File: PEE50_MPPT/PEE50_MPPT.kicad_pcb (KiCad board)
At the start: 2 copper layers, 125 x 125 mm, 174 parts, among them J1 Vout, J2 Conn_01x02_Female, J3 Conn_01x03_Female, J4 Conn_01x03_Female, J5 PV_IN1, J6 PV_IN1, J7 PV_IN1, J8 PV_IN1, Q1 BC547, Q2 BC547, Q3 BC547, Q4 BC547, SW1 SW_DIP_x01, U1 LM3480-3.3, U10 NTA4151PT1G, U11 CSD18514Q5A, U12 CSD18543Q3A, U13 TPS552882QRPMRQ1, U14 MAX44284FAUT+T, U15 MAX44284FAUT+T, U16 NTA4151PT1G, U17 CSD18514Q5A, U18 CSD18543Q3A, U19 TPS552882QRPMRQ1, U2 MSP430FR2353TDBT, U20 MAX44284FAUT+T, U21 MAX44284FAUT+T, U22 NTA4151PT1G, U23 CSD18514Q5A, U24 CSD18543Q3A, U25 TPS552882QRPMRQ1, U26 MAX44284FAUT+T, U27 MAX44284FAUT+T, U3 ADG706BRUZ, U4 NTA4151PT1G, U5 CSD18514Q5A, U6 CSD18543Q3A, U7 TPS552882QRPMRQ1, U8 MAX44284FAUT+T, U9 MAX44284FAUT+T

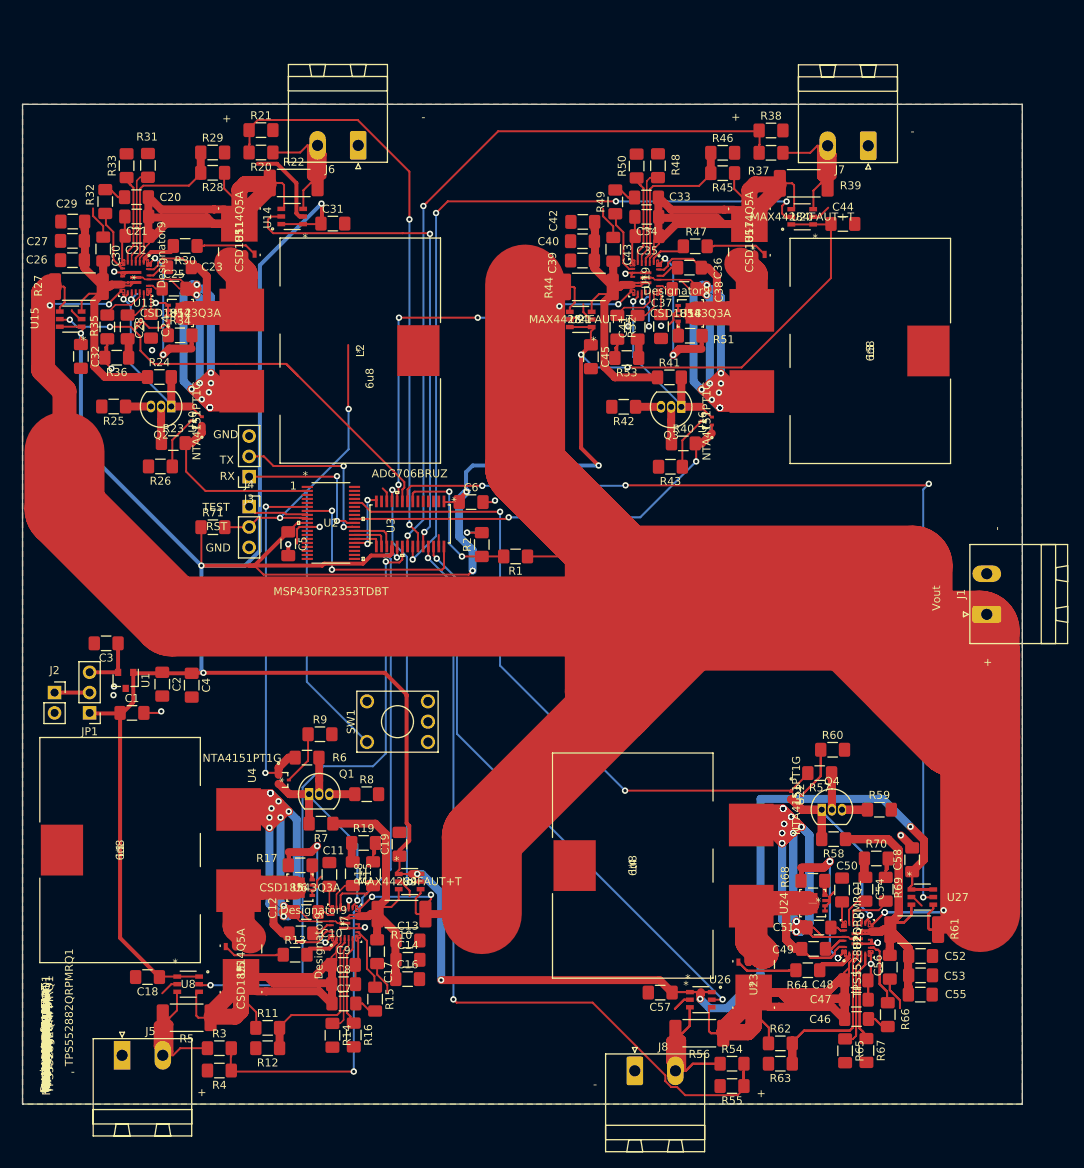
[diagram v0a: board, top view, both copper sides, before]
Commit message: PCB gedecimeert
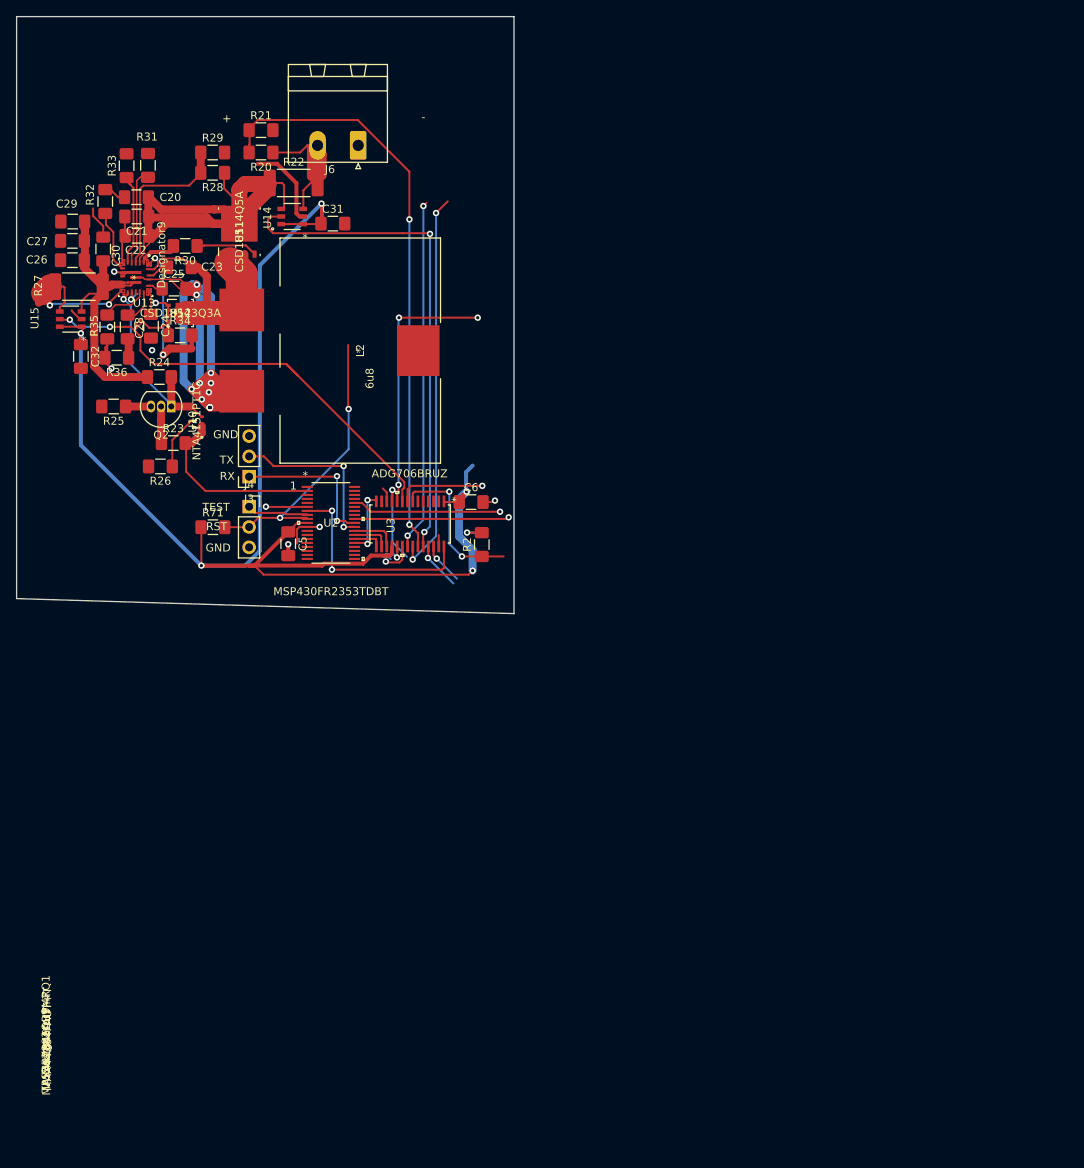
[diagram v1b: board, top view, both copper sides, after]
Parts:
- removed C1, C3: 1u, Capacitor_SMD:C_1206_3216Metric_Pad1.42x1.75mm_HandSolder
- removed C10, C12, C15, C18, C19, C2, C36, C38, C4, C41, C44, C45, C49, C51, C54, C57, C58: 100n, Capacitor_SMD:C_1206_3216Metric_Pad1.42x1.75mm_HandSolder
- removed C11, C37, C50: 4u7, Capacitor_SMD:C_1206_3216Metric_Pad1.42x1.75mm_HandSolder
- removed C13, C14, C35, C39, C40, C48, C52, C53, C9: 10u, Capacitor_SMD:C_1206_3216Metric_Pad1.42x1.75mm_HandSolder
- removed C16, C17, C42, C43, C55, C56: 39u, Capacitor_SMD:C_1206_3216Metric_Pad1.42x1.75mm_HandSolder
- removed C33, C34, C46, C47, C7, C8: 150u, Capacitor_SMD:C_1206_3216Metric_Pad1.42x1.75mm_HandSolder
- removed J1: Vout, Connector_Phoenix_MSTB:PhoenixContact_MSTBA_2,5_2-G-5,08_1x02_P5.08mm_Horizontal
- removed J2: Conn_01x02_Female, Connector_PinSocket_2.54mm:PinSocket_1x02_P2.54mm_Vertical
- removed J5, J7, J8: PV_IN1, Connector_Phoenix_MSTB:PhoenixContact_MSTBA_2,5_2-G-5,08_1x02_P5.08mm_Horizontal
- removed JP1: Jumper_NC_Dual, Connector_PinHeader_2.54mm:PinHeader_1x03_P2.54mm_Vertical
- removed L1, L3, L4: 6u8, AudioProject:SER2915L-153KL
- removed Q1, Q3, Q4: BC547, Package_TO_SOT_THT:TO-92_Inline
- removed R1, R3, R37, R54: 180k, Resistor_SMD:R_1206_3216Metric_Pad1.42x1.75mm_HandSolder
- removed R10, R39, R44, R5, R56, R61: 0.01, Resistor_SMD:R_2512_6332Metric_Pad1.52x3.35mm_HandSolder
- removed R11, R45, R62: 383k, Resistor_SMD:R_1206_3216Metric_Pad1.42x1.75mm_HandSolder
- removed R12, R14, R16, R46, R48, R50, R63, R65, R67: 100k, Resistor_SMD:R_1206_3216Metric_Pad1.42x1.75mm_HandSolder
- removed R13, R17, R47, R51, R64, R68: 1, Resistor_SMD:R_1206_3216Metric_Pad1.42x1.75mm_HandSolder
- removed R15, R49, R66: 66.5k, Resistor_SMD:R_1206_3216Metric_Pad1.42x1.75mm_HandSolder
- removed R18, R52, R69: 21k, Resistor_SMD:R_1206_3216Metric_Pad1.42x1.75mm_HandSolder
- removed R19, R53, R70: 13k, Resistor_SMD:R_1206_3216Metric_Pad1.42x1.75mm_HandSolder
- removed R38, R4, R55: 20k, Resistor_SMD:R_1206_3216Metric_Pad1.42x1.75mm_HandSolder
- removed R40, R42, R43, R57, R59, R6, R60, R8, R9: R, Resistor_SMD:R_1206_3216Metric_Pad1.42x1.75mm_HandSolder
- removed R41, R58, R7: 10k, Resistor_SMD:R_1206_3216Metric_Pad1.42x1.75mm_HandSolder
- removed SW1: SW_DIP_x01, Button_Switch_THT:KSA_Tactile_SPST
- removed U1: LM3480-3.3, Package_TO_SOT_SMD:SOT-23
- removed U16, U22, U4: NTA4151PT1G, AudioProject:NTA4151PT1G
- removed U17, U23, U5: CSD18514Q5A, Robin_Lib:DQJ0008A
- removed U18, U24, U6: CSD18543Q3A, Robin_Lib:DNH0008A
- removed U19, U25, U7: TPS552882QRPMRQ1, Robin_Lib:RPM0026A-MFG
- removed U20, U21, U26, U27, U8, U9: MAX44284FAUT+T, Robin_Lib:21-0058I_MXM
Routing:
- net /Sheet609B465C/Vout: track 495.2 -> 19.7 mm, vias 9 -> 2
- net +3V3: track 522.4 -> 188.3 mm, vias 13 -> 5
- net Net-(C51-Pad2): track 189.4 -> 0.00 mm, vias 26 -> 0
- net /sheet609F5795/sheet609C6964/PVin+: track 138.4 -> 0.00 mm
- net Pgnd: track 183.9 -> 57.9 mm, vias 24 -> 9
- net Imppt4: track 120.2 -> 11.0 mm, vias 4 -> 1
- net Vpv4: track 106.1 -> 5.96 mm, vias 2 -> 1
- net Net-(C38-Pad2): track 94.7 -> 0.00 mm, vias 13 -> 0
- net Net-(C12-Pad2): track 94.7 -> 0.00 mm, vias 13 -> 0
- net Vpv1: track 88.7 -> 4.42 mm, vias 2 -> 1
- net /sheet609F5795/sheet609C6964/ISP: track 79.7 -> 0.00 mm
- net Ipv1: track 77.4 -> 3.91 mm, vias 2 -> 1
- net /sheet609F4756/sheet609C6964/PVin+: track 69.2 -> 0.00 mm
- net /Sheet609B465C/sheet609C6964/PVin+: track 69.2 -> 0.00 mm
- net Ipv4: track 72.9 -> 5.25 mm, vias 2 -> 1
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- removed copper zone on B.Cu, net Pgnd
- removed copper zone on F.Cu, net Pgnd
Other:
- board size 125 x 125 mm -> 62.2 x 74.6 mm
- board text removed: "Vout"
